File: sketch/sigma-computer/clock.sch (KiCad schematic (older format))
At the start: 7 parts

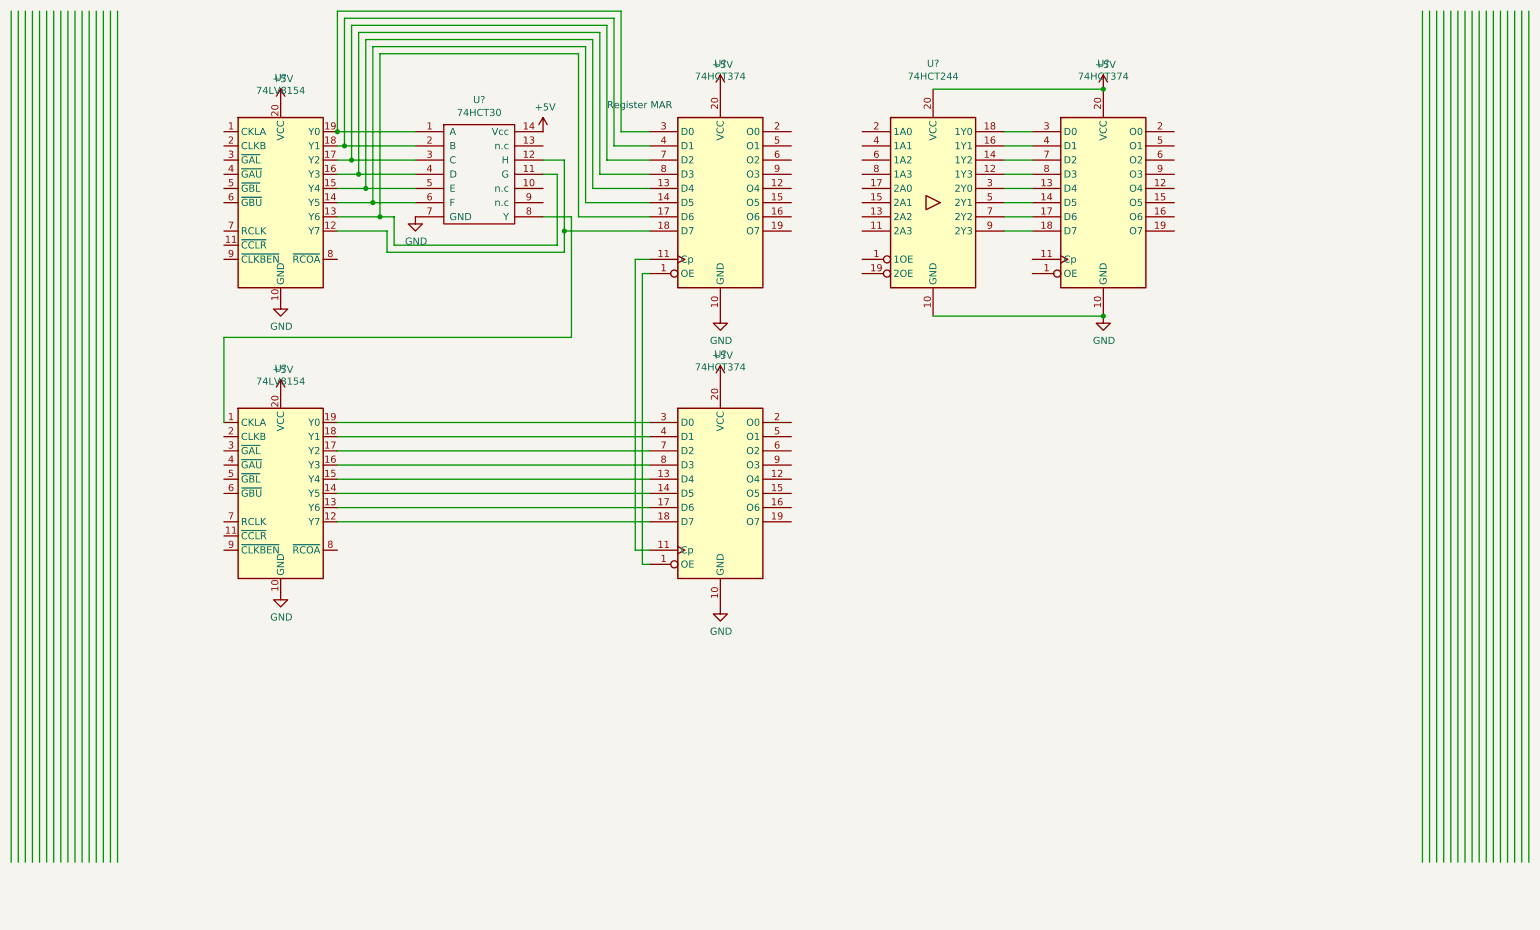
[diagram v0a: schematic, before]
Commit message: Changes in the schematic
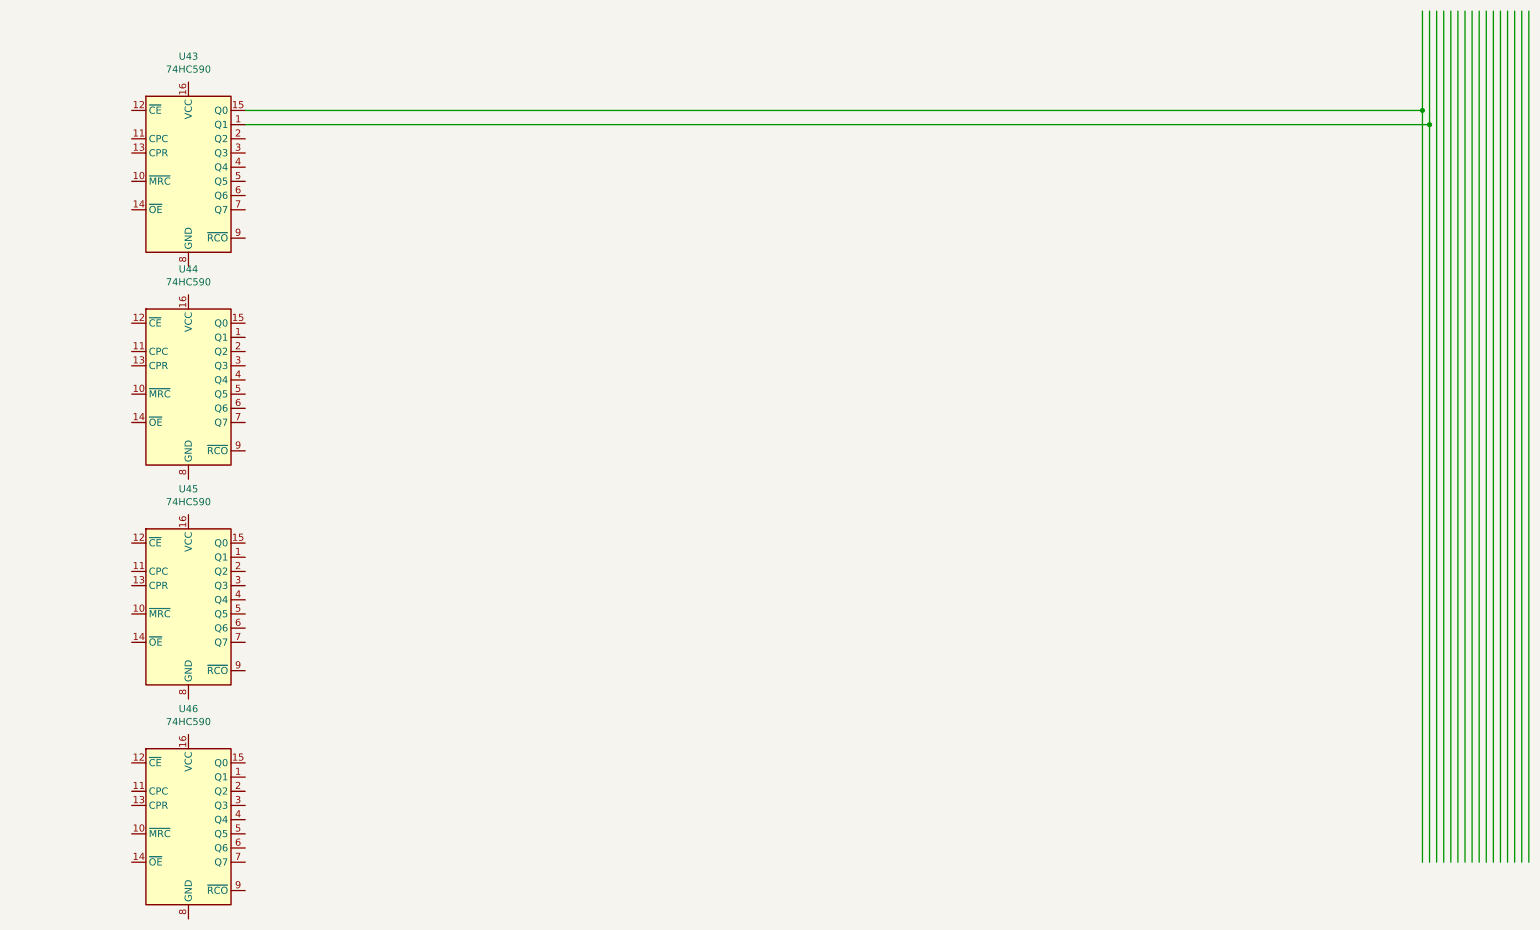
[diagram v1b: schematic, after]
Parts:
- removed U?: 74LV8154, symbol 74xx:74LV8154
- removed U? (x3): 74HCT374, symbol 74xx:74HCT374
- removed U?: 74LV8154, symbol 74HC253:74LV8154
- removed U?: 74HCT30, symbol Additional74:74HCT30
- removed U?: 74HCT244, symbol 74xx:74HCT244
- added U43, U44, U45, U46: 74HC590, symbol 74HC253:74HC590
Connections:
- net labels removed: +5V, GND
- wire segments 112 -> 20
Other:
- note removed: "Register MAR"
